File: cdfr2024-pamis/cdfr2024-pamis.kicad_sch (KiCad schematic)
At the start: 24 parts, among them J1 Connecteur batterie, J14 Conn_ST_STDC14, J4 Connecteur Programmation, J5 Connecteur Débug, J5 Connecteur ToF, J6 Moteur Droit, J7 Moteur Gauche, U1 LM317_SOT-223, U1 STM32F401RCTx, U4 Driver Moteur Droit, U5 Driver Moteur Gauche

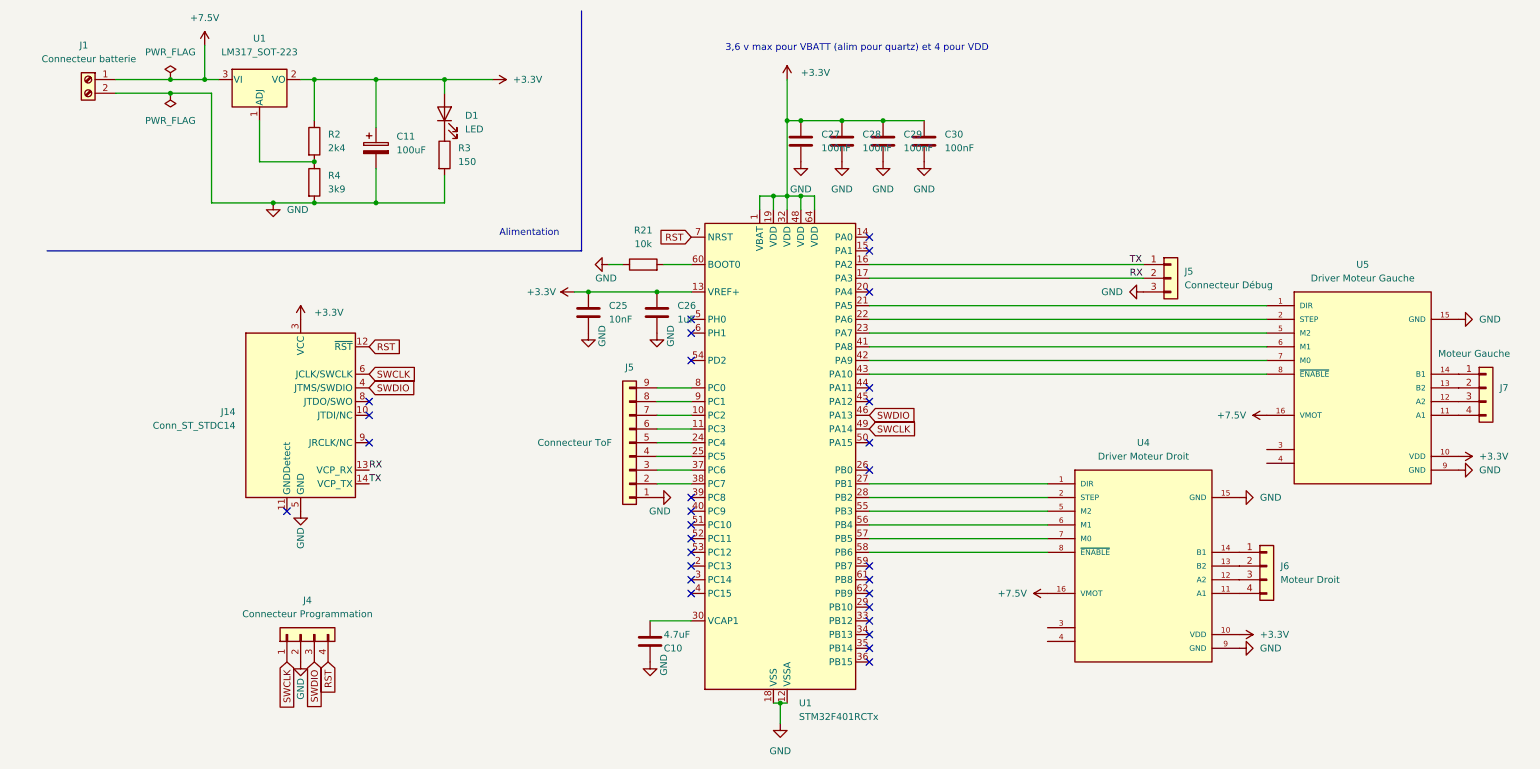
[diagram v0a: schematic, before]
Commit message: module wifi
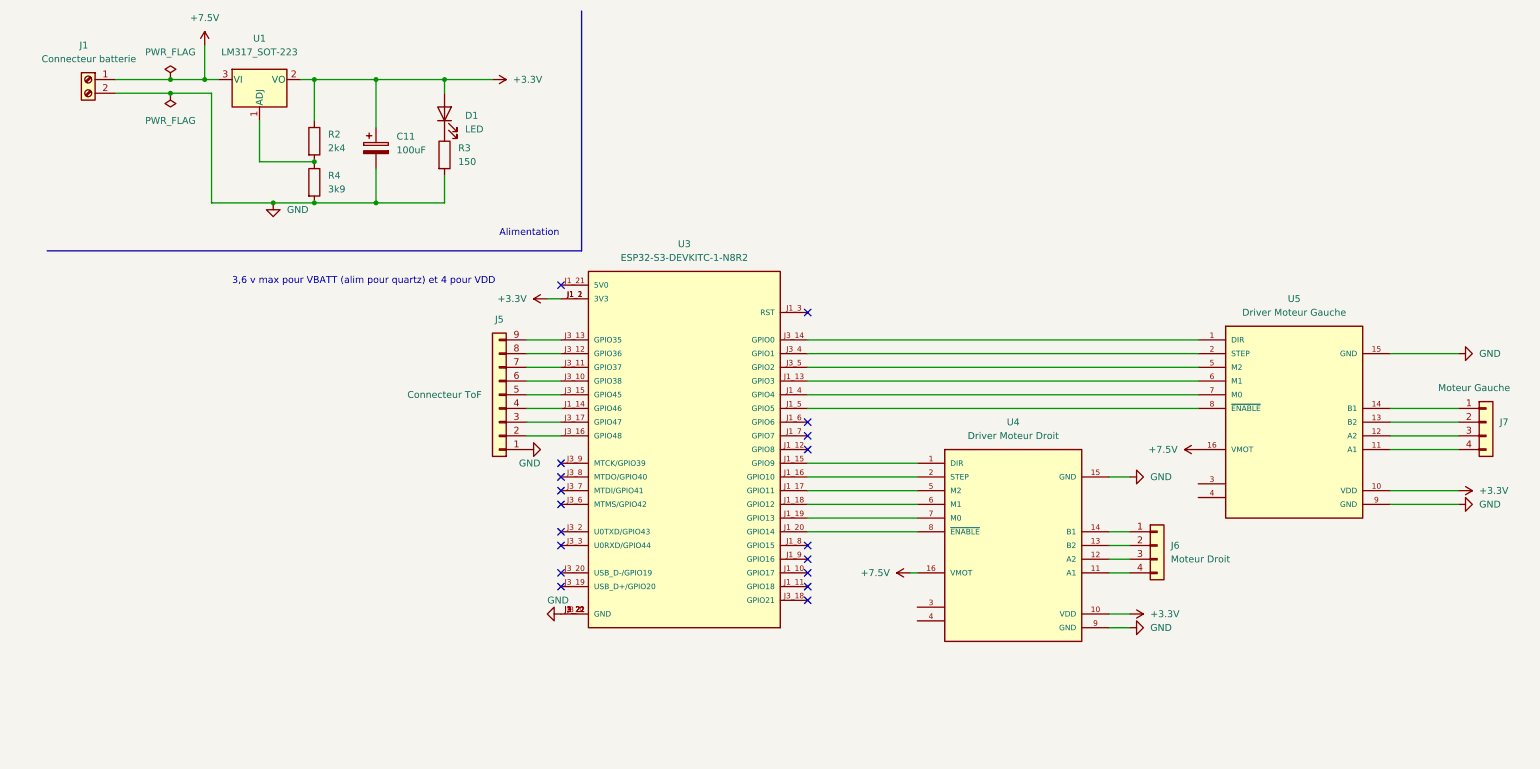
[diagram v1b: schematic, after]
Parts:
- removed C10: 4.7uF, Capacitor_SMD:C_0805_2012Metric_Pad1.18x1.45mm_HandSolder, symbol Device:C
- removed C25: 10nF, Capacitor_SMD:C_0805_2012Metric_Pad1.18x1.45mm_HandSolder, symbol Device:C
- removed C26: 1uF, Capacitor_SMD:C_0805_2012Metric_Pad1.18x1.45mm_HandSolder, symbol Device:C
- removed C27, C28, C29, C30: 100nF, Capacitor_SMD:C_0805_2012Metric_Pad1.18x1.45mm_HandSolder, symbol Device:C
- removed J14: Conn_ST_STDC14, FTSH-107-01-L-DV-K-A:SAMTEC_FTSH-107-01-L-DV-K-A, symbol Connector:Conn_ST_STDC14
- removed J4: Connecteur Programmation, Connector_PinHeader_2.54mm:PinHeader_1x04_P2.54mm_Vertical, symbol Connector_Generic:Conn_01x04
- removed J5: Connecteur Débug, Connector_PinHeader_2.54mm:PinHeader_1x03_P2.54mm_Vertical, symbol Connector_Generic:Conn_01x03
- removed R21: 10k, Resistor_SMD:R_0805_2012Metric_Pad1.20x1.40mm_HandSolder, symbol Device:R
- removed U1: STM32F401RCTx, Package_QFP:LQFP-64_10x10mm_P0.5mm, symbol MCU_ST_STM32F4:STM32F401RCTx
- added U3: ESP32-S3-DEVKITC-1-N8R2, ESP32S3-devkit:ESP32-S3-DEVKITC, symbol ESP32-S3-DEVKITC-1-N8R2:ESP32-S3-DEVKITC-1-N8R2
- U4, U5: footprint A4988_Stepper_Motor_Driver:MODULE_A4988_STEPPER_MOTOR_DRIVER_CARRIER -> A4988:MODULE_A4988_STEPPER_MOTOR_DRIVER_CARRIER
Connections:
- net +3.3V: now also U3.J1_1 (3V3), U3.J1_2 (3V3)
- net GND: now also U3.J1_22 (GND), U3.J3_1 (GND), U3.J3_21 (GND), U3.J3_22 (GND)
- net at U4.1 (DIR): now also U3.J1_15 (GPIO9)
- net at U4.2 (STEP): now also U3.J1_16 (GPIO10)
- net at U4.5 (M2): now also U3.J1_17 (GPIO11)
- net at U4.6 (M1): now also U3.J1_18 (GPIO12)
- net at U4.7 (M0): now also U3.J1_19 (GPIO13)
- net at U4.8 (~{ENABLE}): now also U3.J1_20 (GPIO14)
- net at J5.7 (Pin_7): now also U3.J3_11 (GPIO37)
- net at J5.6 (Pin_6): now also U3.J3_10 (GPIO38)
- net at U5.1 (DIR): now also U3.J3_14 (GPIO0)
- net at U5.2 (STEP): now also U3.J3_4 (GPIO1)
- net at U5.5 (M2): now also U3.J3_5 (GPIO2)
- net at J5.5 (Pin_5): now also U3.J3_15 (GPIO45)
- net at J5.4 (Pin_4): now also U3.J1_14 (GPIO46)
- net at J5.3 (Pin_3): now also U3.J3_17 (GPIO47)
- net at J5.2 (Pin_2): now also U3.J3_16 (GPIO48)
- net at U5.6 (M1): now also U3.J1_13 (GPIO3)
- net at U5.7 (M0): now also U3.J1_4 (GPIO4)
- net at U5.8 (~{ENABLE}): now also U3.J1_5 (GPIO5)
- net at J5.9 (Pin_9): now also U3.J3_13 (GPIO35)
- net at J5.8 (Pin_8): now also U3.J3_12 (GPIO36)
- no-connect marks 30 -> 18
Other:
- moved on the sheet: J5, J6, J7, U4, U5
